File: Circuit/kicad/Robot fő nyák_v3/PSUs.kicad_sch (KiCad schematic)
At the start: 70 parts, among them U31 AP64501SP-13, U32 AP64501SP-13, U33 AP64501SP-13, U34 AP64501SP-13, U35 AP64501SP-13

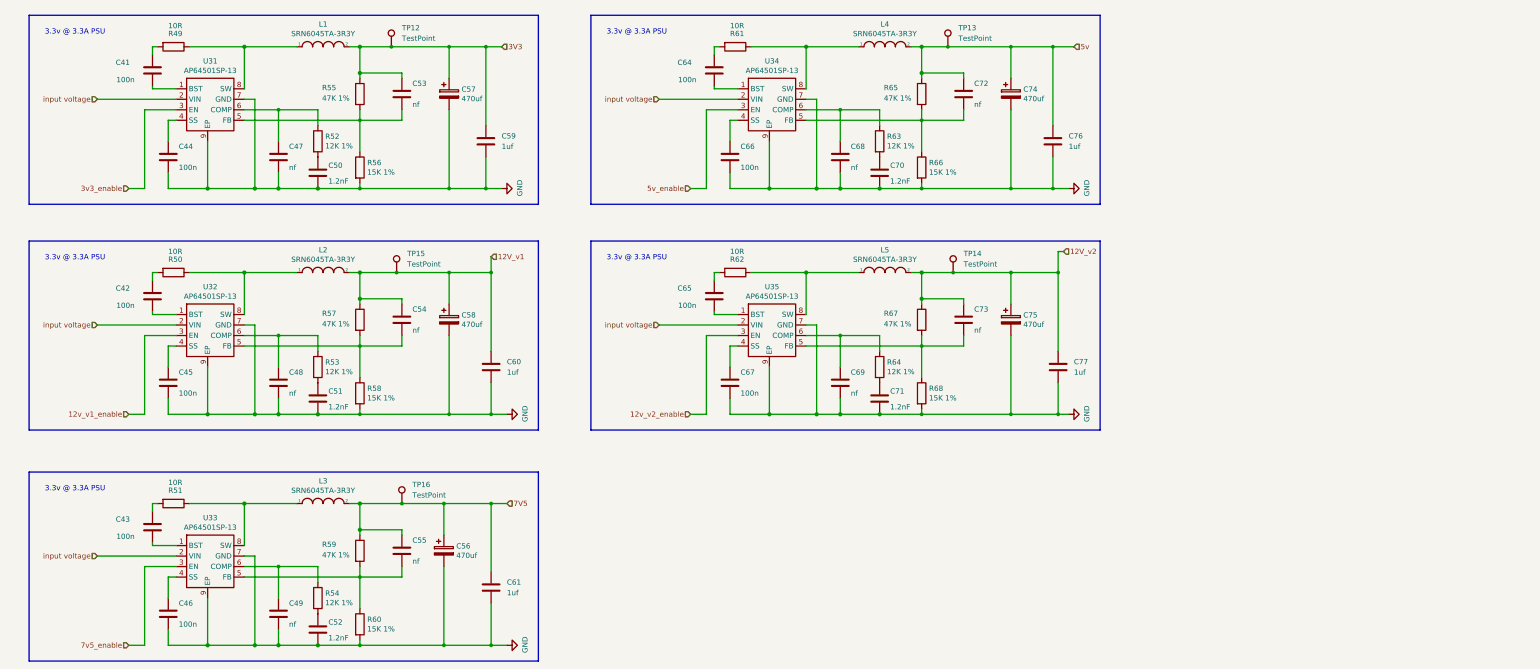
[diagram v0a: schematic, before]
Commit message: updated kicad (big_update)
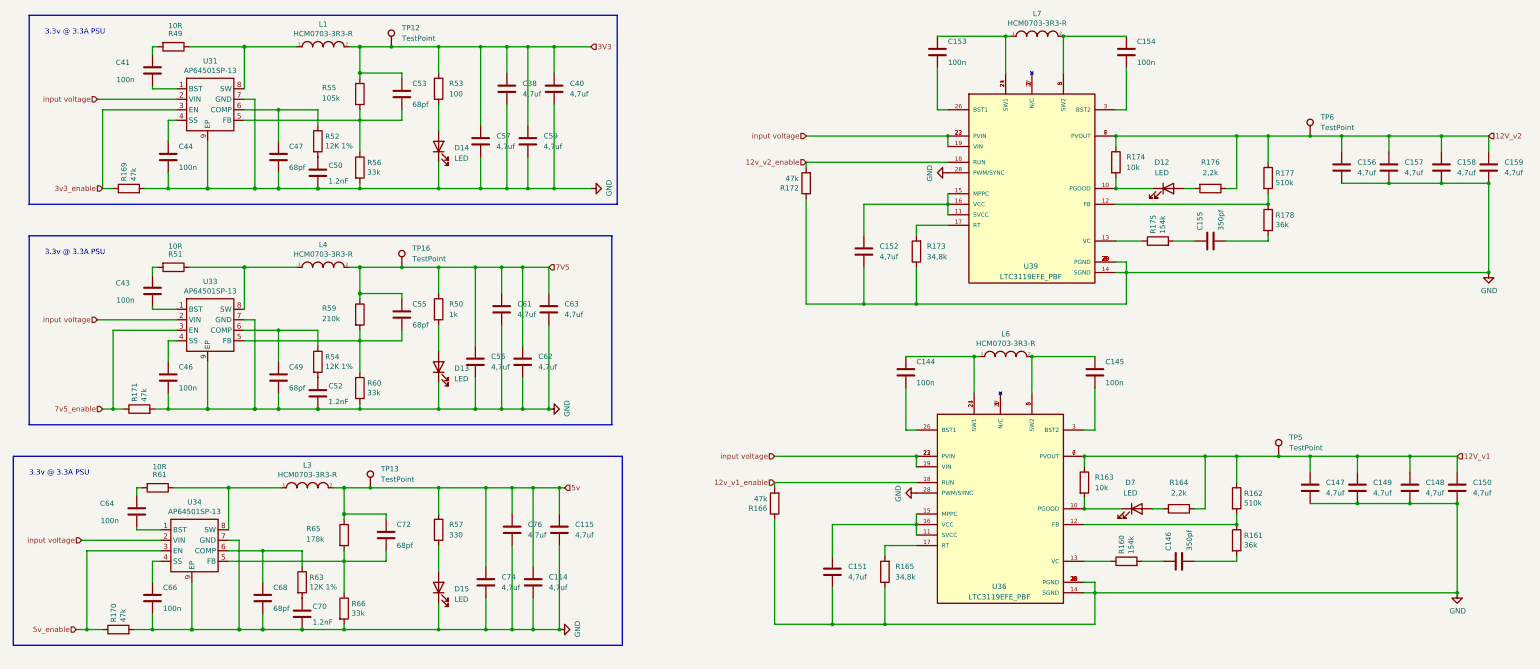
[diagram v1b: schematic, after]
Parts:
- removed C42, C45, C65, C67: 100n, Capacitor_SMD:C_0805_2012Metric, symbol Device:C
- removed C48, C54, C69, C73: nf, Capacitor_SMD:C_0805_2012Metric, symbol Device:C
- removed C51, C71: 1.2nF, Capacitor_SMD:C_0805_2012Metric, symbol Device:C
- removed C56, C57, C58, C74, C75: 470uf, Capacitor_SMD:CP_Elec_8x10, symbol Device:CP
- removed C60, C77: 1uf, Capacitor_SMD:C_0805_2012Metric, symbol Device:C
- removed L2, L5: SRN6045TA-3R3Y, Inductor_SMD:L_Bourns_SRN6045TA, symbol pspice:INDUCTOR
- removed R58, R68: 15K 1%, Resistor_SMD:R_0805_2012Metric, symbol Device:R
- removed R62: 10R, Resistor_SMD:R_0805_2012Metric, symbol Device:R
- removed R64: 12K 1%, Resistor_SMD:R_0805_2012Metric, symbol Device:R
- removed R67: 47K 1%, Resistor_SMD:R_0805_2012Metric, symbol Device:R
- removed TP14, TP15: TestPoint, TestPoint:TestPoint_Pad_D2.0mm, symbol Connector:TestPoint
- removed U32, U35: AP64501SP-13, Package_SO:SOIC-8-1EP_3.9x4.9mm_P1.27mm_EP2.95x4.9mm_Mask2.71x3.4mm_ThermalVias, symbol CM4IO:AP64351
- added C114, C115, C147, C148, C149, C150, C151, C152, C156, C157, C158, C159, C38, C40, C56, C57, C62, C63, C74: 4,7uf, Capacitor_SMD:C_0805_2012Metric, symbol Device:C
- added C144, C145, C153, C154: 100n, Capacitor_SMD:C_0805_2012Metric, symbol Device:C
- added C146, C155: 350pf, Capacitor_SMD:C_0805_2012Metric, symbol Device:C
- added D12, D13, D14, D15, D7: LED, Diode_SMD:D_1206_3216Metric, symbol Device:LED
- added L6, L7: HCM0703-3R3-R, Inductor_SMD:L_KOHERelec_MDA7030, symbol pspice:INDUCTOR
- added R160, R175: 154k, Resistor_SMD:R_0805_2012Metric, symbol Device:R
- added R161, R178: 36k, Resistor_SMD:R_0805_2012Metric, symbol Device:R
- added R162, R177: 510k, Resistor_SMD:R_0805_2012Metric, symbol Device:R
- added R163, R174: 10k, Resistor_SMD:R_0805_2012Metric, symbol Device:R
- added R164, R176: 2,2k, Resistor_SMD:R_0805_2012Metric, symbol Device:R
- added R165, R173: 34,8k, Resistor_SMD:R_0805_2012Metric, symbol Device:R
- added R166, R169, R170, R171, R172: 47k, Resistor_SMD:R_0805_2012Metric, symbol Device:R
- added TP5, TP6: TestPoint, TestPoint:TestPoint_Pad_D2.0mm, symbol Connector:TestPoint
- added U36, U39: LTC3119EFE_PBF, CM5IO:SOP65P640X120-29N, symbol LTC3119EFE_PBF:LTC3119EFE_PBF
- C47, C49, C53, C55, C68, C72: value nf -> 68pf
- C59, C61, C76: value 1uf -> 4,7uf
- L1, L3, L4: value SRN6045TA-3R3Y -> HCM0703-3R3-R; footprint Inductor_SMD:L_Bourns_SRN6045TA -> Inductor_SMD:L_KOHERelec_MDA7030
- R50: value 10R -> 1k; Field4 Farnell -> (none); Field5 9238999 -> (none); Field6 RC0402FR-0710RL -> (none); Field7 Yageo -> (none); Field8 URES00256 -> (none); Part Description Resistor 10R M1005 1% 63mW -> (none)
- R53: value 12K 1% -> 100; Field4 Farnell -> (none); Field5 9239367 -> (none); Field6 MCR01MZPF1202 -> (none); Field7 Rohm -> (none); Part Description Resistor 12K M1005 1% 63mW -> (none)
- R55: value 47K 1% -> 105k
- R56, R60, R66: value 15K 1% -> 33k
- R57: value 47K 1% -> 330; Field4 Farnell -> (none); Field5 9239430 -> (none); Field6 RK73G1ETQTP4702D -> (none); Field7 KOA EUROPE GMBH -> (none); Field8 120892781 -> (none); Part Description Resistor 47K M1005 1% 63mW -> (none)
- R59: value 47K 1% -> 210k
- R65: value 47K 1% -> 178k
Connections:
- net 12V_v1: now also C147.1, C148.1, C149.1, C150.1, R162.1, R163.1, R164.1, TP5.1, U36.6 (PVOUT), U36.7 (PVOUT); no longer R57.1
- net 12V_v2: now also C156.1, C157.1, C158.1, C159.1, R174.1, R176.1, R177.1, TP6.1, U39.6 (PVOUT), U39.7 (PVOUT)
- net 12v_v1_enable: now also R166.2, U36.18 (RUN)
- net 12v_v2_enable: now also R172.2, U39.18 (RUN)
- net 3V3: now also R53.1, C38.1, C40.1, C57.1
- net 3v3_enable: now also R169.1
- net 5v: now also L3.2, R57.1, C114.1, C115.1, C74.1; no longer L4.2
- net 5v_enable: now also R170.1
- net 7V5: now also L4.2, R50.1, C56.1, C62.1, C63.1; no longer L3.2
- net 7v5_enable: now also R171.1
- net GND: now also C114.2, C115.2, C147.2, C148.2, C149.2, C150.2, C151.2, C152.2, C156.2, C157.2, C158.2, C159.2, C38.2, C40.2, C56.2, C57.2, C62.2, C63.2, C74.2, D13.1 (K), D14.1 (K), D15.1 (K), R165.1, R166.1, R169.2, R170.2, R171.2, R172.1, R173.1, U36.14 (SGND), U36.20 (PGND), U36.25 (PGND), U36.28 (PWM/SYNC), U36.29 (PGND), U36.4 (PGND), U36.9 (PGND), U39.14 (SGND), U39.20 (PGND), U39.25 (PGND), U39.28 (PWM/SYNC), U39.29 (PGND), U39.4 (PGND), U39.9 (PGND)
- net input voltage: now also U36.19 (VIN), U36.22 (PVIN), U36.23 (PVIN), U39.19 (VIN), U39.22 (PVIN), U39.23 (PVIN)
- net at R51.1, U33.8 (SW): now also L4.1; no longer L3.1
- net at R57.2: now also D15.2 (A)
- net at R50.2: now also D13.2 (A)
- net at R61.1, U34.8 (SW): now also L3.1; no longer L4.1
- net at R53.2: now also D14.2 (A)
- new net: R165.2, U36.17 (RT)
- new net: C146.1, R160.2
- new net: C146.2, R161.2
- new net: C145.1, L6.2, U36.5 (SW2), U36.8 (SW2)
- new net: C145.2, U36.3 (BST2)
- new net: C155.1, R175.2
- new net: C155.2, R178.2
- new net: D7.1 (K), R163.2, U36.10 (PGOOD)
- new net: R161.1, R162.2, U36.12 (FB)
- new net: C144.1, L6.1, U36.21 (SW1), U36.24 (SW1)
- new net: C144.2, U36.26 (BST1)
- new net: D12.2 (A), R176.2
- new net: C153.1, L7.1, U39.21 (SW1), U39.24 (SW1)
- new net: C154.1, L7.2, U39.5 (SW2), U39.8 (SW2)
- new net: U36.1 (N/C), U36.2 (N/C), U36.27 (N/C)
- new net: C151.1, U36.11 (SVCC), U36.15 (MPPC), U36.16 (VCC)
- new net: R160.1, U36.13 (VC)
- new net: D7.2 (A), R164.2
- new net: R177.2, R178.1, U39.12 (FB)
- new net: C153.2, U39.26 (BST1)
- new net: D12.1 (K), R174.2, U39.10 (PGOOD)
- new net: R175.1, U39.13 (VC)
- new net: U39.1 (N/C), U39.2 (N/C), U39.27 (N/C)
- new net: C152.1, U39.11 (SVCC), U39.15 (MPPC), U39.16 (VCC)
- new net: R173.2, U39.17 (RT)
- new net: C154.2, U39.3 (BST2)
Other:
- moved on the sheet: C43, C46, C49, C52, C55, C59, C64, C66, C68, C70, C72, R51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
